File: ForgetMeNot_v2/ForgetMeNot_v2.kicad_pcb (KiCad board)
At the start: 4 copper layers, 22.3 x 32.6 mm, 44 parts, among them J1 Conn_01x04, SW1 SW_Push, U1 RP2040, U2 W25Q128JVS, U3 NCP1117, U4 LIS2HH12, U5 MCP1640x-xMC, Y1 Crystal_ABM8

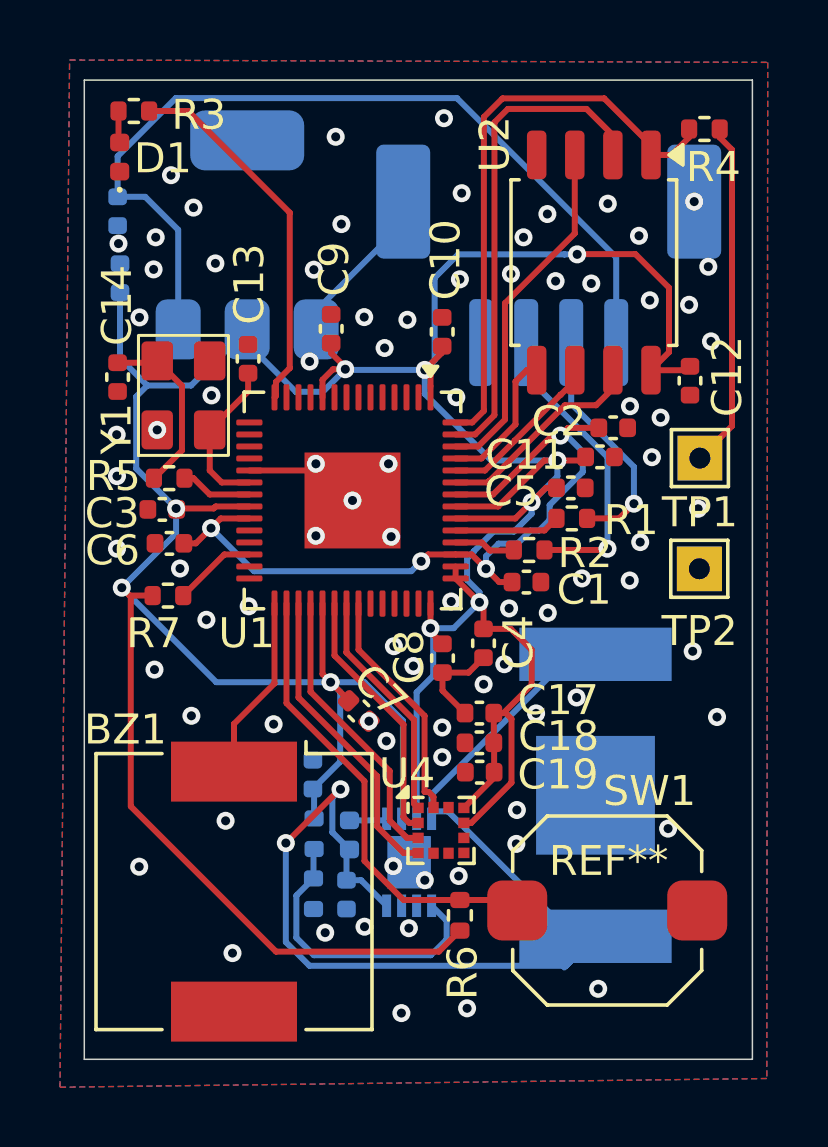
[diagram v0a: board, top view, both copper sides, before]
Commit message: finished layout & tracing
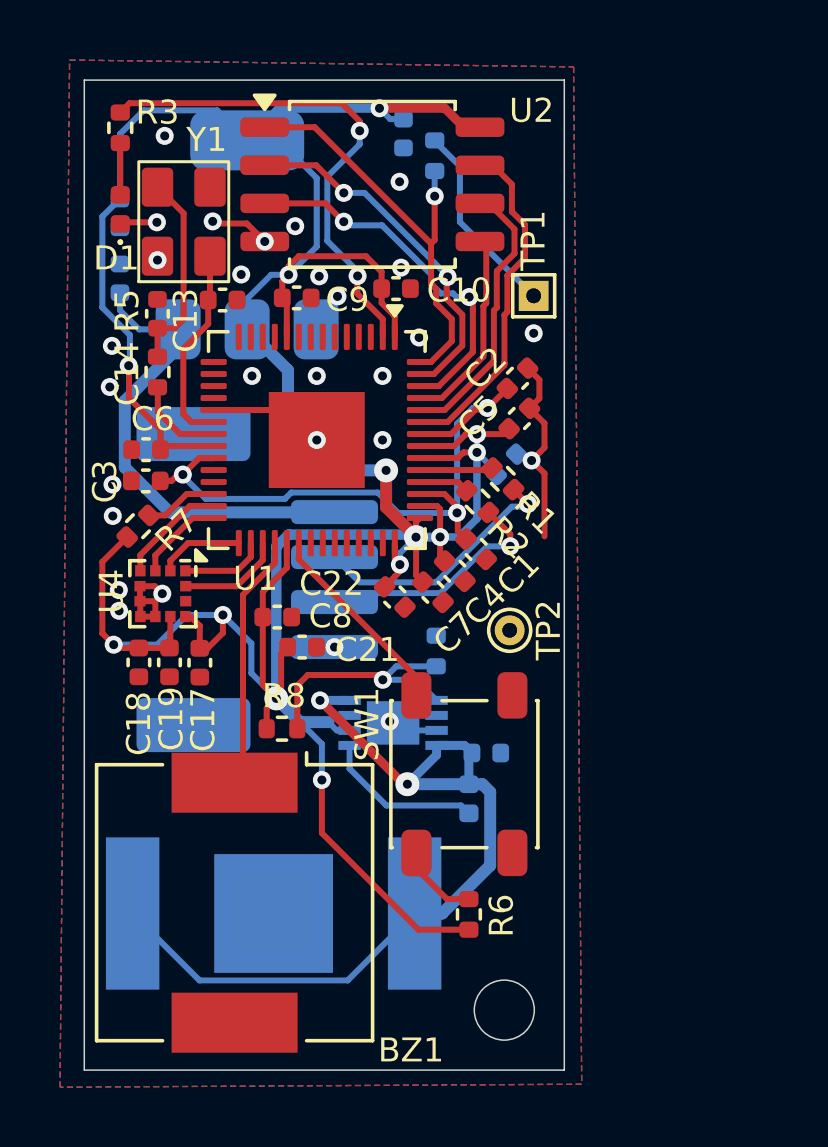
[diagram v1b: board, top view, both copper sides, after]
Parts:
- added C22: 100n, Capacitor_SMD:C_0402_1005Metric, F.Cu at (141.0, 95.5)
- C11, C12, R4: moved to B.Cu
- C21, R8: moved to F.Cu
- SW1: footprint Button_Switch_SMD:SW_Push_1TS009xxxx-xxxx-xxxx_6x6x5mm -> Button_Switch_SMD:SW_SPST_PTS647_Sx38
- TP1: footprint TestPoint:TestPoint_THTPad_1.5x1.5mm_Drill0.7mm -> TestPoint:TestPoint_THTPad_1.0x1.0mm_Drill0.5mm
- TP2: footprint TestPoint:TestPoint_THTPad_1.5x1.5mm_Drill0.7mm -> TestPoint:TestPoint_THTPad_D1.0mm_Drill0.5mm
- moved J1 14.3 mm to (136.4, 94.9), turned to 90 degrees
- moved C12 12.6 mm to (141.3, 80.0)
- moved U4 12.2 mm to (133.3, 95.4), turned to -90 degrees
- moved C18 11.7 mm to (132.5, 97.7), turned to 90 degrees
- moved BT1 11.4 mm to (137.0, 106.0), turned to 0 degrees
- moved C19 11.0 mm to (133.5, 97.7), turned to 90 degrees
- moved C17 9.47 mm to (134.5, 97.7), turned to 90 degrees
- moved R9 9.07 mm to (142.4, 97.3), turned to 90 degrees
- moved R4 9.03 mm to (142.3, 80.8), turned to -90 degrees
- moved U2 7.83 mm to (140.3, 81.7), turned to 0 degrees
- moved TP1 7.74 mm to (145.6, 85.4)
- moved TP2 6.64 mm to (144.8, 96.6)
- moved C20 6.63 mm to (144.1, 100.7), turned to 0 degrees
- moved SW1 6.58 mm to (143.3, 101.4), turned to 90 degrees
- moved Y1 5.79 mm to (134.0, 83.0)
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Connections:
- U1 pad 14: /LED -> unconnected-(U1-GPIO11-Pad14)
- U1 pad 2: unconnected-(U1-GPIO0-Pad2) -> /LED
- U1 pad 27: unconnected-(U1-GPIO16-Pad27) -> /ACC_SDA
- U1 pad 28: unconnected-(U1-GPIO17-Pad28) -> /ACC_SDO
- U1 pad 29: /BUZZ -> /ACC_CS
- U1 pad 30: /ZERO -> /ACC_SCL
- U1 pad 31: /ACC_SDA -> /ACC_INT
- U1 pad 32: /ACC_SDO -> /BUZZ
- U1 pad 34: /ACC_CS -> /ZERO
- U1 pad 35: /ACC_SCL -> unconnected-(U1-GPIO23-Pad35)
- U1 pad 36: /ACC_INT -> unconnected-(U1-GPIO24-Pad36)
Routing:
- net +5V: track 29.6 -> 15.7 mm
- net +3.3V: track 137.8 -> 127.1 mm, vias 10 -> 13
- net Net-(BT1-+): track 38.9 -> 28.9 mm
- net GND: track 11.2 -> 21.0 mm, vias 83 -> 28
- net /ZERO: track 15.8 -> 8.63 mm
- net /ACC_SDA: track 10.2 -> 3.65 mm
- net /ACC_SDO: track 9.51 -> 2.98 mm
- net /ACC_CS: track 8.64 -> 2.86 mm
- net Net-(R4-Pad1): track 11.6 -> 6.55 mm
- net /ACC_SCL: track 7.80 -> 2.84 mm
- net /QSPI_SS: track 19.5 -> 14.7 mm, vias 0 -> 1
- net /QSPI_SD1: track 16.5 -> 12.0 mm, vias 0 -> 2
- net /ACC_INT: track 7.91 -> 3.49 mm
- net /LED: track 12.5 -> 16.8 mm, vias 0 -> 2
- net /QSPI_SD3: track 7.15 -> 11.4 mm
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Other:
- board size 22.3 x 32.6 mm -> 16 x 33 mm
